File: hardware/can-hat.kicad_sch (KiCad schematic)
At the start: 0 parts

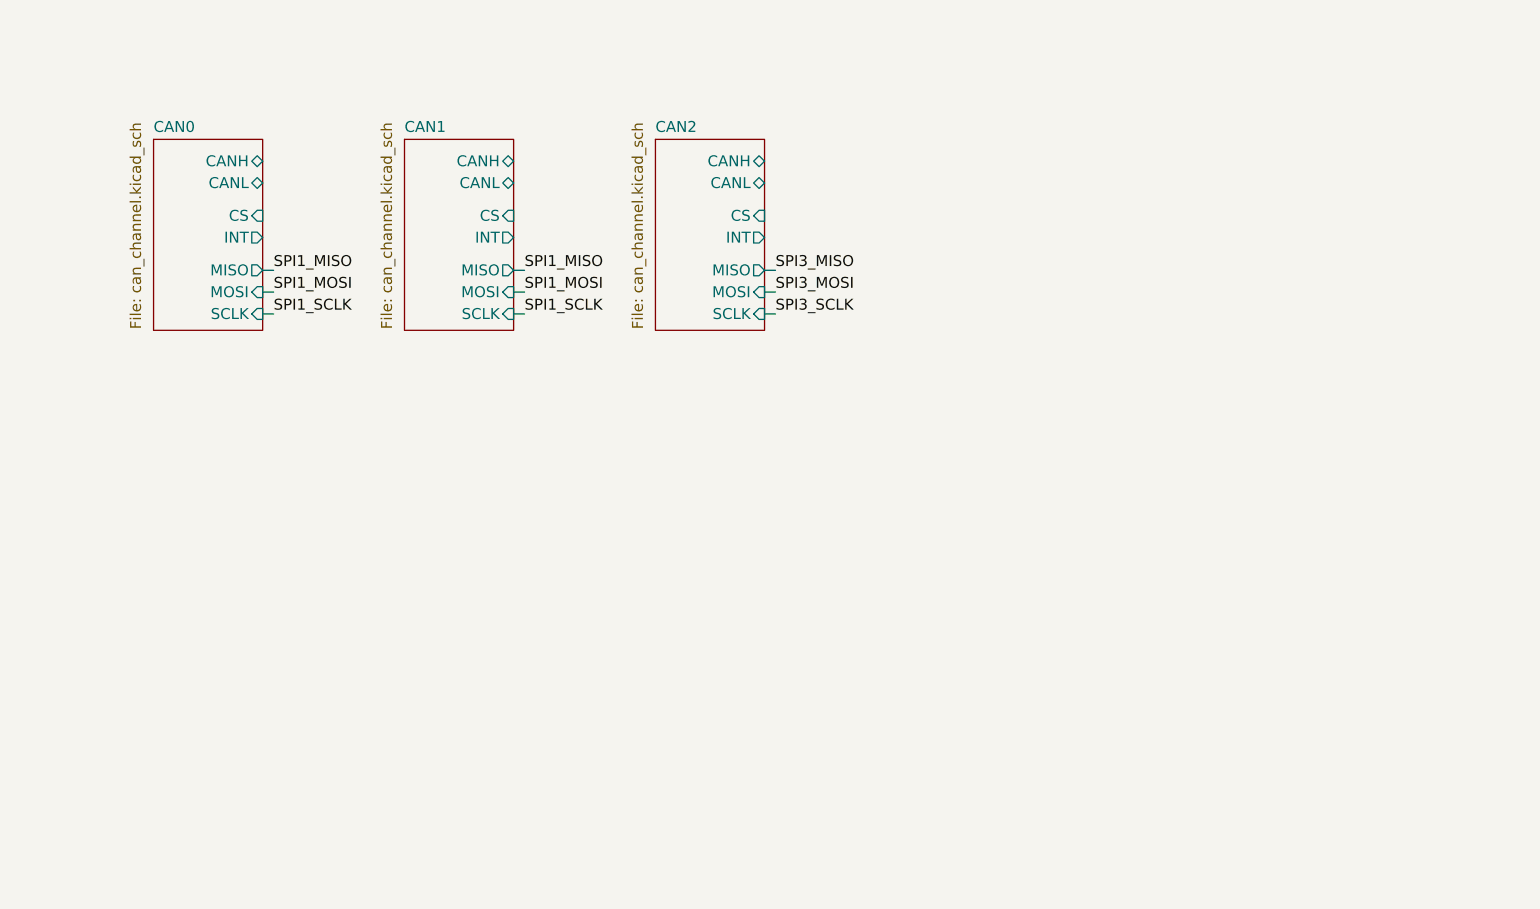
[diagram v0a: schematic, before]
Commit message: feat: finish the schematic
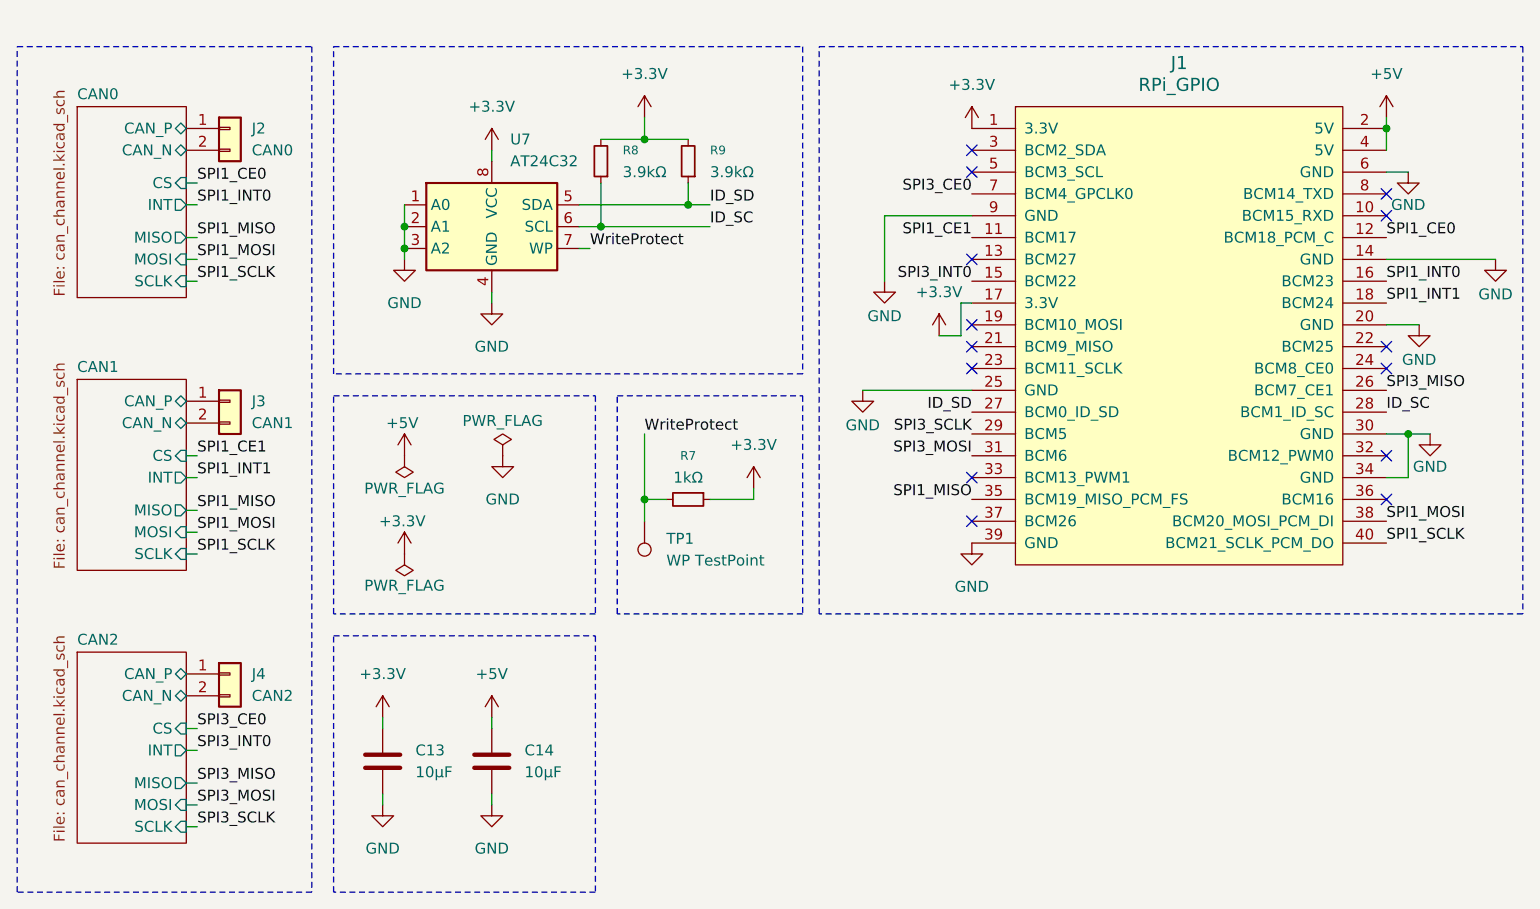
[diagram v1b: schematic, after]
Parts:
- added C13, C14: 10µF, Capacitor_SMD:C_0805_2012Metric, symbol Device:C
- added J1: RPi_GPIO, RPI_Hat:RPI_Hat_B+, symbol RPi_Hat:RPi_GPIO
- added J2: CAN0, Degson:SHDRRA2W80P0X350_1X2_780X920X722P, symbol Connector_Generic:Conn_01x02
- added J3: CAN1, Degson:SHDRRA2W80P0X350_1X2_780X920X722P, symbol Connector_Generic:Conn_01x02
- added J4: CAN2, Degson:SHDRRA2W80P0X350_1X2_780X920X722P, symbol Connector_Generic:Conn_01x02
- added R7: 1kΩ, Resistor_SMD:R_0201_0603Metric, symbol Device:R_Small
- added R8, R9: 3.9kΩ, Resistor_SMD:R_0201_0603Metric, symbol Device:R_Small
- added TP1: WP TestPoint, TestPoint:TestPoint_Pad_1.5x1.5mm, symbol Connector:TestPoint
- added U7: AT24C32, Package_SO:SOIC-8_3.9x4.9mm_P1.27mm, symbol Memory_EEPROM:24C02Cx-x-SN
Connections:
- net SPI1_MISO: now also J1.35 (BCM19_MISO_PCM_FS)
- net SPI1_MOSI: now also J1.38 (BCM20_MOSI_PCM_DI)
- net SPI1_SCLK: now also J1.40 (BCM21_SCLK_PCM_DO)
- net SPI3_MISO: now also J1.26 (BCM7_CE1)
- net SPI3_MOSI: now also J1.31 (BCM6)
- net SPI3_SCLK: now also J1.29 (BCM5)
- new net +3.3V: C13.1, J1.1 (3.3V), J1.17 (3.3V), R7.1, R8.2, R9.2, U7.8 (VCC)
- new net +5V: C14.1, J1.2 (5V), J1.4 (5V)
- new net CAN0/CAN_N: J2.2 (Pin_2)
- new net CAN0/CAN_P: J2.1 (Pin_1)
- new net CAN1/CAN_N: J3.2 (Pin_2)
- new net CAN1/CAN_P: J3.1 (Pin_1)
- new net CAN2/CAN_N: J4.2 (Pin_2)
- new net CAN2/CAN_P: J4.1 (Pin_1)
- new net GND: C13.2, C14.2, J1.14 (GND), J1.20 (GND), J1.25 (GND), J1.30 (GND), J1.34 (GND), J1.39 (GND), J1.6 (GND), J1.9 (GND), U7.1 (A0), U7.2 (A1), U7.3 (A2), U7.4 (GND)
- new net ID_SC: J1.28 (BCM1_ID_SC), R8.1, U7.6 (SCL)
- new net ID_SD: J1.27 (BCM0_ID_SD), R9.1, U7.5 (SDA)
- new net SPI1_CE0: J1.12 (BCM18_PCM_C)
- new net SPI1_CE1: J1.11 (BCM17)
- new net SPI1_INT0: J1.16 (BCM23)
- new net SPI1_INT1: J1.18 (BCM24)
- new net SPI3_CE0: J1.7 (BCM4_GPCLK0)
- new net SPI3_INT0: J1.15 (BCM22)
- new net WriteProtect: R7.2, TP1.1, U7.7 (WP)
- no-connect marks 0 -> 14
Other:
- sheet CAN0 ports: added CAN_N, CAN_P; removed CANH, CANL
- sheet CAN1 ports: added CAN_N, CAN_P; removed CANH, CANL
- sheet CAN2 ports: added CAN_N, CAN_P; removed CANH, CANL
- company: (none) -> Kieran Klukas
- title: (none) -> CAN Hat
